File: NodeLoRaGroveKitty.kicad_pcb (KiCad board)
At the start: 2 copper layers, 50 x 50 mm, 42 parts, among them IC1 CP2104, P1 PICKIT PROGRAMMER, P2 Battery, P3 USB_B, P4 A0, P5 D9, P6 I2C, Q1 MMBT2222A, Q2 MMBT2222A, SW1 SW_RESET, U1 AP2114, U2 MCP73831T-2ATI/OT, U3 ESP8266-12E

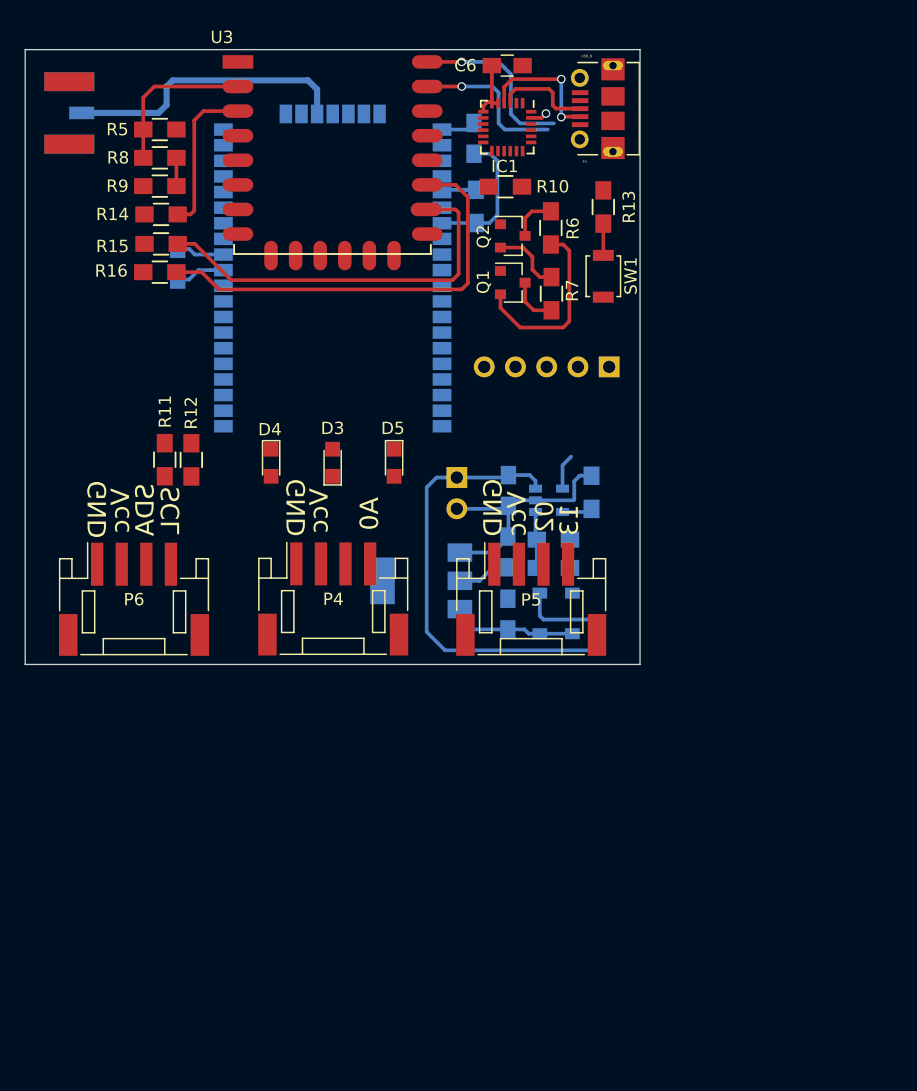
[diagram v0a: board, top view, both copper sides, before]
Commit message: PCB 1.0v
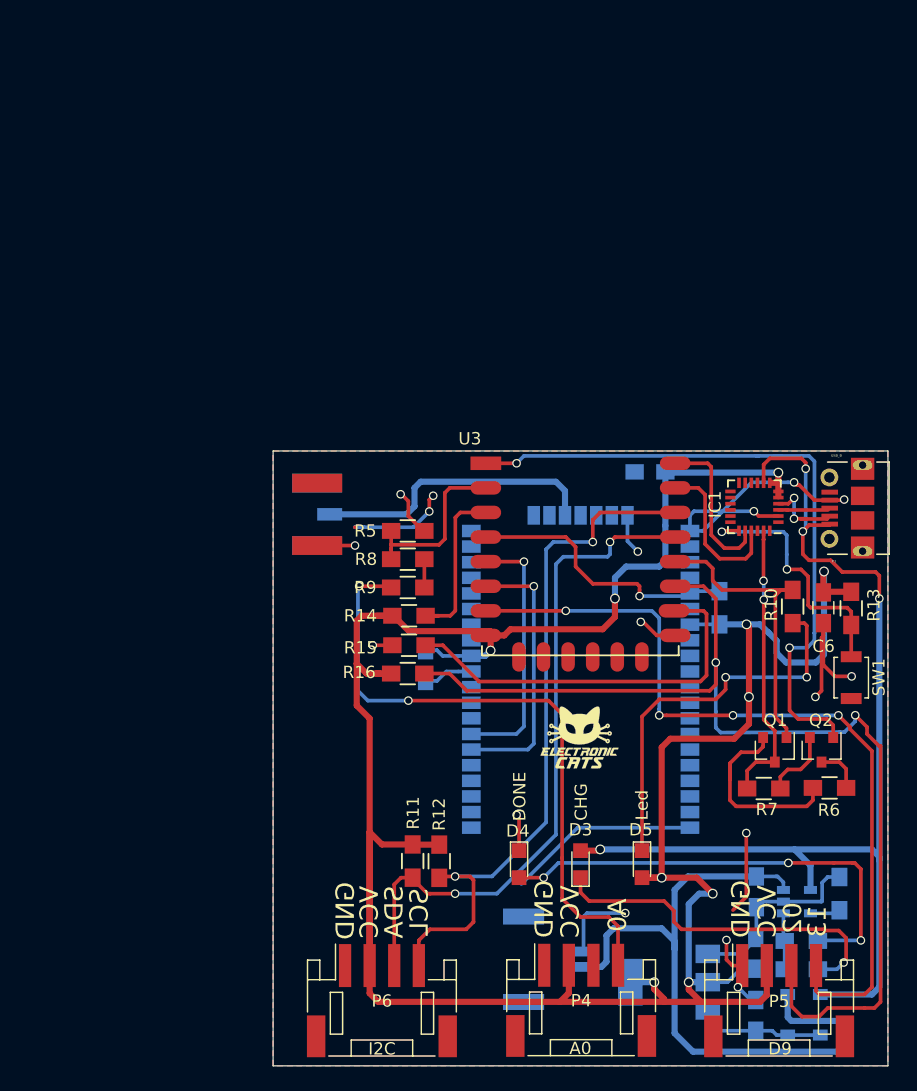
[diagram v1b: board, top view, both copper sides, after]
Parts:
- removed P1: PICKIT PROGRAMMER, Pin_Headers:Pin_Header_Straight_1x05_Pitch2.54mm
- added G***: LOGO, modules:electronic_cats_logo_4x3, F.Cu at (145.1, 105.9)
- P2: footprint Pin_Headers:Pin_Header_Angled_1x02_Pitch2.54mm -> modules:panelmate_smd_2
- moved C6 51.0 mm to (164.9, 95.4), turned to 270 degrees
- moved R6 50.9 mm to (165.4, 110.0), turned to 0 degrees
- moved Q2 48.8 mm to (164.8, 106.9), turned to 270 degrees
- moved R7 43.8 mm to (160.1, 110.1), turned to 180 degrees
- moved Q1 43.6 mm to (161.0, 106.9), turned to 270 degrees
- moved R10 41.4 mm to (162.4, 95.3), turned to 270 degrees
- moved P2 39.8 mm to (141.9, 124.0), turned to 90 degrees
- moved R14 38.4 mm to (131.2, 96.0)
- moved U1 38.4 mm to (152.4, 125.8)
- moved A1 38.4 mm to (121.7, 87.8)
- moved D1 38.4 mm to (164.7, 128.5)
- moved D2 38.4 mm to (162.0, 128.5)
- moved P4 38.4 mm to (145.2, 127.3)
- moved R13 38.4 mm to (167.2, 95.4)
- moved R15 38.4 mm to (131.2, 98.4)
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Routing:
- net +3V3: track 24.2 -> 226.9 mm, vias 0 -> 10
- net VCC: track 2.89 -> 91.3 mm, vias 0 -> 4
- net GND: track 27.8 -> 102.4 mm, vias 0 -> 14
- net /GPIO13: track 0.00 -> 66.5 mm, vias 0 -> 4
- net /SCL: track 0.00 -> 57.0 mm, vias 0 -> 2
- net /SDA: track 0.00 -> 55.1 mm, vias 0 -> 2
- net /RESET: track 0.00 -> 54.2 mm, vias 0 -> 2
- net /GPIO2: track 35.9 -> 89.2 mm, vias 0 -> 2
- net /A0: track 0.00 -> 52.2 mm, vias 0 -> 2
- net Net-(D4-Pad2): track 0.07 -> 37.9 mm, vias 0 -> 3
- net Net-(D5-Pad1): track 0.00 -> 31.6 mm, vias 0 -> 2
- net Net-(D3-Pad1): track 0.00 -> 29.3 mm, vias 0 -> 1
- net /GPIO0: track 0.00 -> 25.3 mm
- net /SRX: track 0.00 -> 21.3 mm, vias 0 -> 1
- net /STX: track 0.00 -> 20.3 mm, vias 0 -> 1
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- added copper zone on B.Cu, net GND
- added copper zone on F.Cu, net GND
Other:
- board text added: "VCC"
- board text removed: "Vcc"
